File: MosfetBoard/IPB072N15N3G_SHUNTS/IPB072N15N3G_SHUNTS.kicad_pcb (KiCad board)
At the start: 2 copper layers, 125 x 75 mm, 112 parts, among them J1 DRIVER1, J13 BATT+Conn2, J14 BATT-Conn2, J15 PHASE_PAD, J16 PHASE_PAD, J2 DRIVER1, J3 DRIVER1, J4 PhaseConn, J5 PhaseConn, J6 PhaseConn, J7 PHASE_PAD, J8 BATT+Conn1, J9 BATT-Conn1, Q1 IPB072N15N3G, Q10 IPB072N15N3G, Q11 IPB072N15N3G, Q12 IPB072N15N3G, Q2 IPB072N15N3G, Q3 IPB072N15N3G, Q4 IPB072N15N3G, Q5 IPB072N15N3G, Q6 IPB072N15N3G, Q7 IPB072N15N3G, Q8 IPB072N15N3G, Q9 IPB072N15N3G, U1 RS2166XC5, U4 NCS2003ASN2T1G, U5 RS2166XC5, U7 RS2166XC5, U8 NCS2003ASN2T1G, U9 NCS2003ASN2T1G

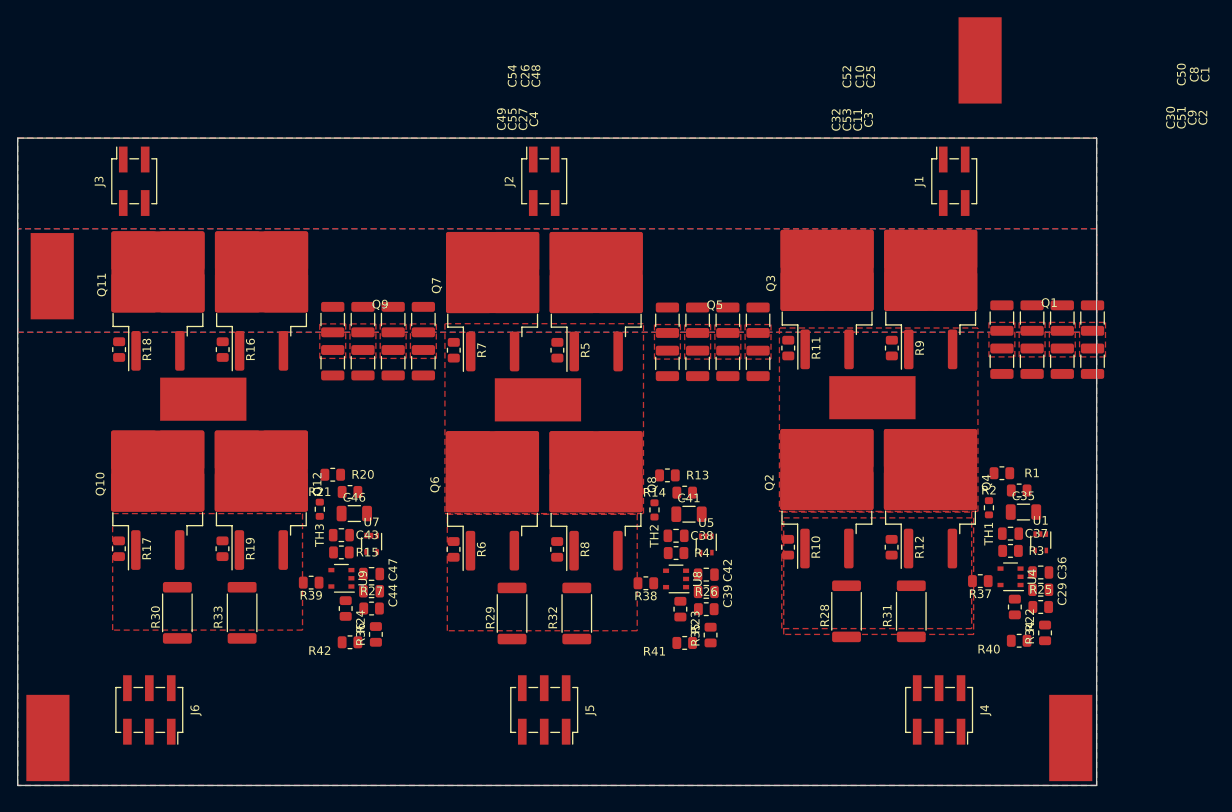
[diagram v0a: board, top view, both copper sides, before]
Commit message: fixeddimensions
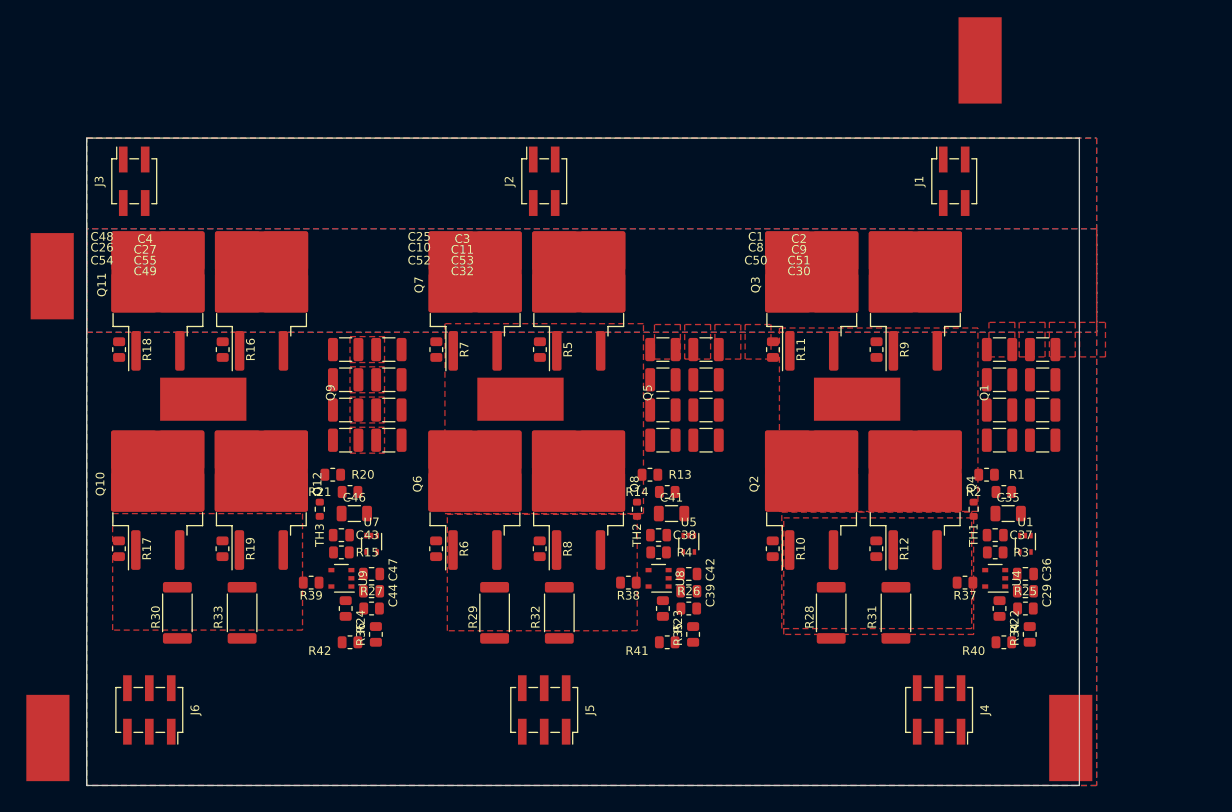
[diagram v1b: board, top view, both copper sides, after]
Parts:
- moved C28 14.2 mm to (208.8, 88.0), turned to 0 degrees
- moved C33 14.1 mm to (133.0, 88.0), turned to 0 degrees
- moved C31 13.9 mm to (169.8, 88.0), turned to 0 degrees
- moved C25 11.5 mm to (169.8, 77.5), turned to 0 degrees
- moved C1 11.4 mm to (208.8, 77.5), turned to 0 degrees
- moved C50 11.3 mm to (208.8, 84.5), turned to 0 degrees
- moved C52 11.2 mm to (169.8, 84.5), turned to 0 degrees
- moved C49 11.1 mm to (138.0, 88.0), turned to 0 degrees
- moved C54 10.7 mm to (133.0, 84.5), turned to 0 degrees
- moved C30 10.3 mm to (213.8, 88.0), turned to 0 degrees
- moved C10 10.2 mm to (169.8, 81.0), turned to 0 degrees
- moved C8 10.2 mm to (208.8, 81.0), turned to 0 degrees
- moved C32 9.96 mm to (174.8, 88.0), turned to 0 degrees
- moved C48 9.65 mm to (133.0, 77.5), turned to 0 degrees
- moved C26 8.88 mm to (133.0, 81.0), turned to 0 degrees
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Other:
- board size 125 x 75 mm -> 115 x 75 mm

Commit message: movedconnectors
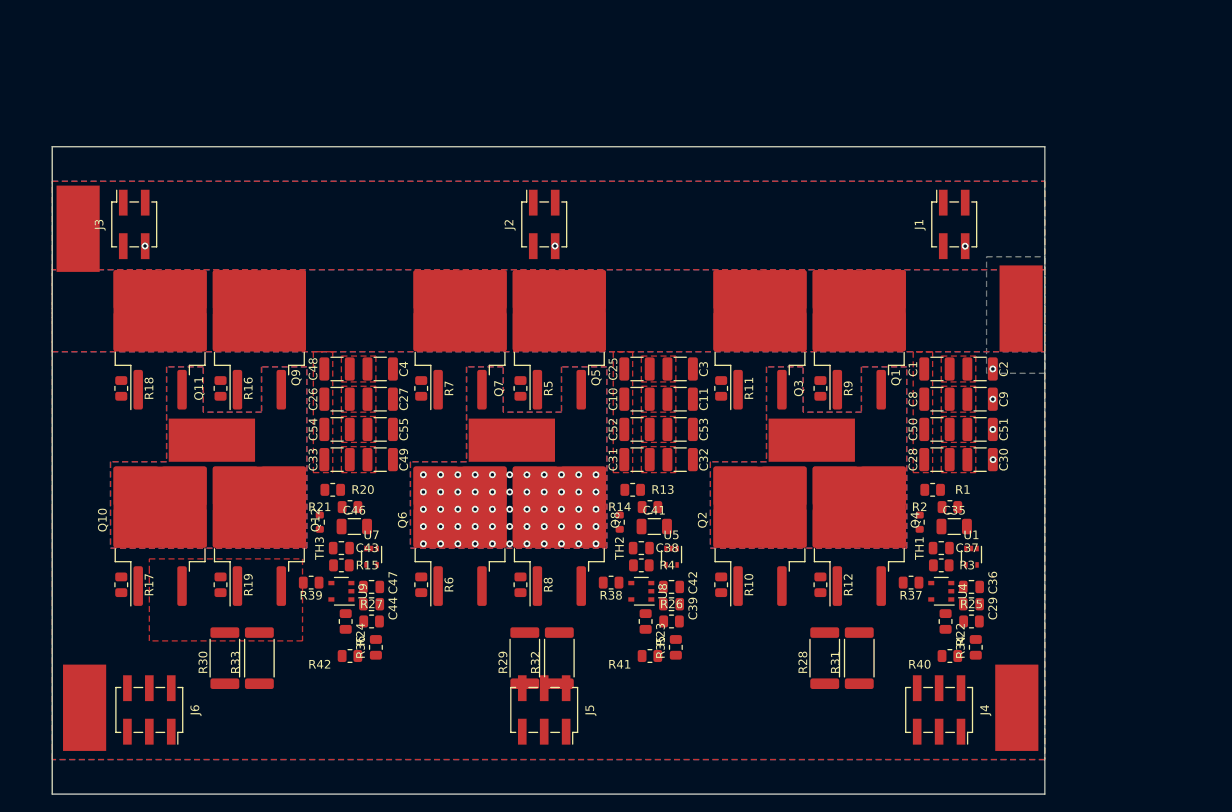
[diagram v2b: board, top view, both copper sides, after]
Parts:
- moved J13 29.1 mm to (211.2, 72.8)
- moved Q1 7.91 mm to (192.5, 74.5)
- moved R9 7.91 mm to (188.0, 82.0)
- moved Q4 7.70 mm to (192.5, 97.2)
- moved R12 7.70 mm to (188.0, 104.8)
- moved R30 7.60 mm to (119.0, 113.2)
- moved C50 7.59 mm to (201.5, 86.8)
- moved C2 7.59 mm to (206.5, 79.8)
- moved C30 7.59 mm to (206.5, 90.2)
- moved C51 7.59 mm to (206.5, 86.8)
- moved C8 7.59 mm to (201.5, 83.2)
- moved C9 7.59 mm to (206.5, 83.2)
- moved C28 7.59 mm to (201.5, 90.2)
- moved C1 7.59 mm to (201.5, 79.8)
- moved Q3 7.50 mm to (181.0, 74.5)
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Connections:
- C29 pad 1: /PhaseMosfets/3.3V_IN -> /PhaseMosfets1/3.3V_IN
- C35 pad 1: /PhaseMosfets/V_SENSE -> /PhaseMosfets1/V_SENSE
- C36 pad 1: /PhaseMosfets/3.3V_IN -> /PhaseMosfets1/3.3V_IN
- C37 pad 1: /PhaseMosfets/MOS_TEMP -> /PhaseMosfets1/MOS_TEMP
- C38 pad 1: /PhaseMosfets1/MOS_TEMP -> /PhaseMosfets2/MOS_TEMP
- C39 pad 1: /PhaseMosfets1/3.3V_IN -> /PhaseMosfets2/3.3V_IN
- C41 pad 1: /PhaseMosfets1/V_SENSE -> /PhaseMosfets2/V_SENSE
- C42 pad 1: /PhaseMosfets1/3.3V_IN -> /PhaseMosfets2/3.3V_IN
- C43 pad 1: /PhaseMosfets2/MOS_TEMP -> /PhaseMosfets3/MOS_TEMP
- C44 pad 1: /PhaseMosfets2/3.3V_IN -> /PhaseMosfets3/3.3V_IN
- C46 pad 1: /PhaseMosfets2/V_SENSE -> /PhaseMosfets3/V_SENSE
- C47 pad 1: /PhaseMosfets2/3.3V_IN -> /PhaseMosfets3/3.3V_IN
- J1 pad 1: /PhaseMosfets/PH -> /PhaseMosfets1/PH
- J1 pad 2: /PhaseMosfets/PL -> /PhaseMosfets1/PL
- J1 pad 3: /PhaseMosfets/PHASE -> /PhaseMosfets1/PHASE
- J15 pad 1: /PhaseMosfets1/PHASE -> /PhaseMosfets2/PHASE
- J16 pad 1: /PhaseMosfets2/PHASE -> /PhaseMosfets3/PHASE
- J2 pad 1: /PhaseMosfets1/PH -> /PhaseMosfets2/PH
- J2 pad 2: /PhaseMosfets1/PL -> /PhaseMosfets2/PL
- J2 pad 3: /PhaseMosfets1/PHASE -> /PhaseMosfets2/PHASE
- J3 pad 1: /PhaseMosfets2/PH -> /PhaseMosfets3/PH
- J3 pad 2: /PhaseMosfets2/PL -> /PhaseMosfets3/PL
- J3 pad 3: /PhaseMosfets2/PHASE -> /PhaseMosfets3/PHASE
- J4 pad 2: /PhaseMosfets/V_SENSE -> /PhaseMosfets1/V_SENSE
- J4 pad 3: /PhaseMosfets/SENSE_FILTER_EN -> /PhaseMosfets1/SENSE_FILTER_EN
- J4 pad 4: /PhaseMosfets/MOS_TEMP -> /PhaseMosfets1/MOS_TEMP
- J4 pad 5: /PhaseMosfets/3.3V_IN -> /PhaseMosfets1/3.3V_IN
- J4 pad 6: /PhaseMosfets/CURRENT_SENSE -> /PhaseMosfets1/CURRENT_SENSE
- J5 pad 2: /PhaseMosfets1/V_SENSE -> /PhaseMosfets2/V_SENSE
- J5 pad 3: /PhaseMosfets1/SENSE_FILTER_EN -> /PhaseMosfets2/SENSE_FILTER_EN
- J5 pad 4: /PhaseMosfets1/MOS_TEMP -> /PhaseMosfets2/MOS_TEMP
- J5 pad 5: /PhaseMosfets1/3.3V_IN -> /PhaseMosfets2/3.3V_IN
- J5 pad 6: /PhaseMosfets1/CURRENT_SENSE -> /PhaseMosfets2/CURRENT_SENSE
- J6 pad 2: /PhaseMosfets2/V_SENSE -> /PhaseMosfets3/V_SENSE
- J6 pad 3: /PhaseMosfets2/SENSE_FILTER_EN -> /PhaseMosfets3/SENSE_FILTER_EN
- J6 pad 4: /PhaseMosfets2/MOS_TEMP -> /PhaseMosfets3/MOS_TEMP
- J6 pad 5: /PhaseMosfets2/3.3V_IN -> /PhaseMosfets3/3.3V_IN
- J6 pad 6: /PhaseMosfets2/CURRENT_SENSE -> /PhaseMosfets3/CURRENT_SENSE
- J7 pad 1: /PhaseMosfets/PHASE -> /PhaseMosfets1/PHASE
- Q1 pad 3: /PhaseMosfets/PHASE -> /PhaseMosfets1/PHASE
- Q10 pad 2: /PhaseMosfets2/PHASE -> /PhaseMosfets3/PHASE
- Q10 pad 3: /PhaseMosfets2/SH+ -> /PhaseMosfets3/SH+
- Q11 pad 3: /PhaseMosfets2/PHASE -> /PhaseMosfets3/PHASE
- Q12 pad 2: /PhaseMosfets2/PHASE -> /PhaseMosfets3/PHASE
- Q12 pad 3: /PhaseMosfets2/SH+ -> /PhaseMosfets3/SH+
- Q2 pad 2: /PhaseMosfets/PHASE -> /PhaseMosfets1/PHASE
- Q2 pad 3: /PhaseMosfets/SH+ -> /PhaseMosfets1/SH+
- Q3 pad 3: /PhaseMosfets/PHASE -> /PhaseMosfets1/PHASE
- Q4 pad 2: /PhaseMosfets/PHASE -> /PhaseMosfets1/PHASE
- Q4 pad 3: /PhaseMosfets/SH+ -> /PhaseMosfets1/SH+
- Q5 pad 3: /PhaseMosfets1/PHASE -> /PhaseMosfets2/PHASE
- Q6 pad 2: /PhaseMosfets1/PHASE -> /PhaseMosfets2/PHASE
- Q6 pad 3: /PhaseMosfets1/SH+ -> /PhaseMosfets2/SH+
- Q7 pad 3: /PhaseMosfets1/PHASE -> /PhaseMosfets2/PHASE
- Q8 pad 2: /PhaseMosfets1/PHASE -> /PhaseMosfets2/PHASE
- Q8 pad 3: /PhaseMosfets1/SH+ -> /PhaseMosfets2/SH+
- Q9 pad 3: /PhaseMosfets2/PHASE -> /PhaseMosfets3/PHASE
- R1 pad 1: /PhaseMosfets/PHASE -> /PhaseMosfets1/PHASE
- R1 pad 2: /PhaseMosfets/V_SENSE -> /PhaseMosfets1/V_SENSE
- R10 pad 1: /PhaseMosfets/PL -> /PhaseMosfets1/PL
- R11 pad 1: /PhaseMosfets/PH -> /PhaseMosfets1/PH
- R12 pad 1: /PhaseMosfets/PL -> /PhaseMosfets1/PL
- R13 pad 1: /PhaseMosfets1/PHASE -> /PhaseMosfets2/PHASE
- R13 pad 2: /PhaseMosfets1/V_SENSE -> /PhaseMosfets2/V_SENSE
- R14 pad 1: /PhaseMosfets1/V_SENSE -> /PhaseMosfets2/V_SENSE
- R15 pad 1: /PhaseMosfets2/MOS_TEMP -> /PhaseMosfets3/MOS_TEMP
- R16 pad 1: /PhaseMosfets2/PH -> /PhaseMosfets3/PH
- R17 pad 1: /PhaseMosfets2/PL -> /PhaseMosfets3/PL
- R18 pad 1: /PhaseMosfets2/PH -> /PhaseMosfets3/PH
- R19 pad 1: /PhaseMosfets2/PL -> /PhaseMosfets3/PL
- R2 pad 1: /PhaseMosfets/V_SENSE -> /PhaseMosfets1/V_SENSE
- R20 pad 1: /PhaseMosfets2/PHASE -> /PhaseMosfets3/PHASE
- R20 pad 2: /PhaseMosfets2/V_SENSE -> /PhaseMosfets3/V_SENSE
- R21 pad 1: /PhaseMosfets2/V_SENSE -> /PhaseMosfets3/V_SENSE
- R22 pad 2: /PhaseMosfets/CURRENT_SENSE -> /PhaseMosfets1/CURRENT_SENSE
- R23 pad 2: /PhaseMosfets1/CURRENT_SENSE -> /PhaseMosfets2/CURRENT_SENSE
- R24 pad 2: /PhaseMosfets2/CURRENT_SENSE -> /PhaseMosfets3/CURRENT_SENSE
- R28 pad 1: /PhaseMosfets/SH+ -> /PhaseMosfets1/SH+
- R29 pad 1: /PhaseMosfets1/SH+ -> /PhaseMosfets2/SH+
- R3 pad 1: /PhaseMosfets/MOS_TEMP -> /PhaseMosfets1/MOS_TEMP
- R30 pad 1: /PhaseMosfets2/SH+ -> /PhaseMosfets3/SH+
- R31 pad 1: /PhaseMosfets/SH+ -> /PhaseMosfets1/SH+
- R32 pad 1: /PhaseMosfets1/SH+ -> /PhaseMosfets2/SH+
- R33 pad 1: /PhaseMosfets2/SH+ -> /PhaseMosfets3/SH+
- R37 pad 1: /PhaseMosfets/SH+ -> /PhaseMosfets1/SH+
- R38 pad 1: /PhaseMosfets1/SH+ -> /PhaseMosfets2/SH+
- R39 pad 1: /PhaseMosfets2/SH+ -> /PhaseMosfets3/SH+
- R4 pad 1: /PhaseMosfets1/MOS_TEMP -> /PhaseMosfets2/MOS_TEMP
- R40 pad 1: /PhaseMosfets/3.3V_IN -> /PhaseMosfets1/3.3V_IN
- R41 pad 1: /PhaseMosfets1/3.3V_IN -> /PhaseMosfets2/3.3V_IN
- R42 pad 1: /PhaseMosfets2/3.3V_IN -> /PhaseMosfets3/3.3V_IN
- R5 pad 1: /PhaseMosfets1/PH -> /PhaseMosfets2/PH
- R6 pad 1: /PhaseMosfets1/PL -> /PhaseMosfets2/PL
- R7 pad 1: /PhaseMosfets1/PH -> /PhaseMosfets2/PH
- R8 pad 1: /PhaseMosfets1/PL -> /PhaseMosfets2/PL
- R9 pad 1: /PhaseMosfets/PH -> /PhaseMosfets1/PH
- TH1 pad 1: /PhaseMosfets/3.3V_IN -> /PhaseMosfets1/3.3V_IN
- TH1 pad 2: /PhaseMosfets/MOS_TEMP -> /PhaseMosfets1/MOS_TEMP
- TH2 pad 1: /PhaseMosfets1/3.3V_IN -> /PhaseMosfets2/3.3V_IN
- TH2 pad 2: /PhaseMosfets1/MOS_TEMP -> /PhaseMosfets2/MOS_TEMP
- TH3 pad 1: /PhaseMosfets2/3.3V_IN -> /PhaseMosfets3/3.3V_IN
- TH3 pad 2: /PhaseMosfets2/MOS_TEMP -> /PhaseMosfets3/MOS_TEMP
- U1 pad 4: /PhaseMosfets/SENSE_FILTER_EN -> /PhaseMosfets1/SENSE_FILTER_EN
- U1 pad 5: /PhaseMosfets/3.3V_IN -> /PhaseMosfets1/3.3V_IN
- U4 pad 5: /PhaseMosfets/3.3V_IN -> /PhaseMosfets1/3.3V_IN
- U5 pad 4: /PhaseMosfets1/SENSE_FILTER_EN -> /PhaseMosfets2/SENSE_FILTER_EN
- U5 pad 5: /PhaseMosfets1/3.3V_IN -> /PhaseMosfets2/3.3V_IN
- U7 pad 4: /PhaseMosfets2/SENSE_FILTER_EN -> /PhaseMosfets3/SENSE_FILTER_EN
- U7 pad 5: /PhaseMosfets2/3.3V_IN -> /PhaseMosfets3/3.3V_IN
- U8 pad 5: /PhaseMosfets1/3.3V_IN -> /PhaseMosfets2/3.3V_IN
- U9 pad 5: /PhaseMosfets2/3.3V_IN -> /PhaseMosfets3/3.3V_IN
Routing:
- net /PhaseMosfets2/PHASE: vias 0 -> 55
- net -BATT: vias 0 -> 7
- added copper zone on B.Cu, net /PhaseMosfets1/PHASE
- added copper zone on B.Cu, net /PhaseMosfets2/PHASE
- added copper zone on F.Cu, net /PhaseMosfets2/PHASE
- added copper zone on B.Cu, net /PhaseMosfets3/PHASE
- added copper zone on F.Cu, net /PhaseMosfets3/PHASE
- removed copper zone on F.Cu, net /PhaseMosfets/PHASE
- removed copper zone on F.Cu, net /PhaseMosfets/SH+
- removed copper zone on F.Cu, net /PhaseMosfets1/SH+
